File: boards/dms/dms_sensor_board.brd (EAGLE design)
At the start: 49.5 x 44.5 mm, 33 parts, among them Q1 IRLML5203, Q2 IRLML5203, Q3 IRLML5203, Q4 IRLML5203

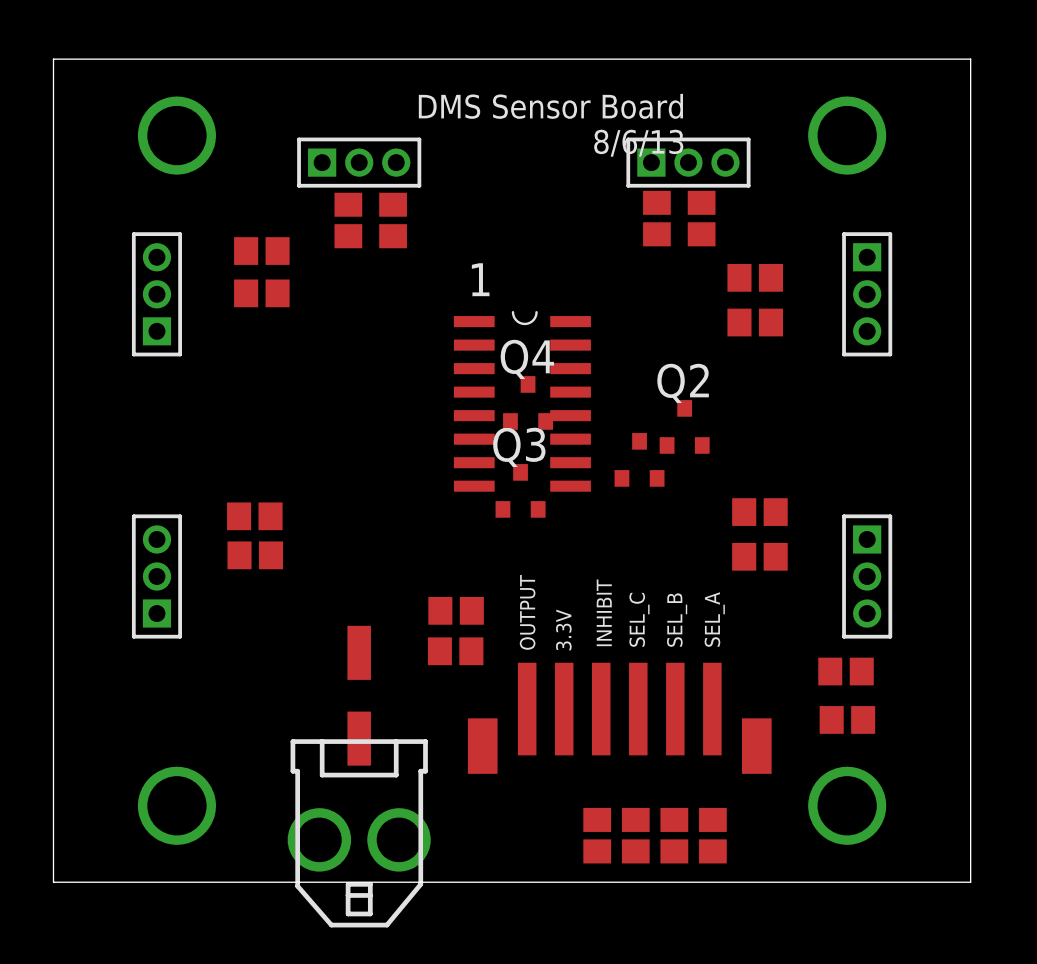
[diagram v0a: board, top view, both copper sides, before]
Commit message: changes for new boards, cleared DRC
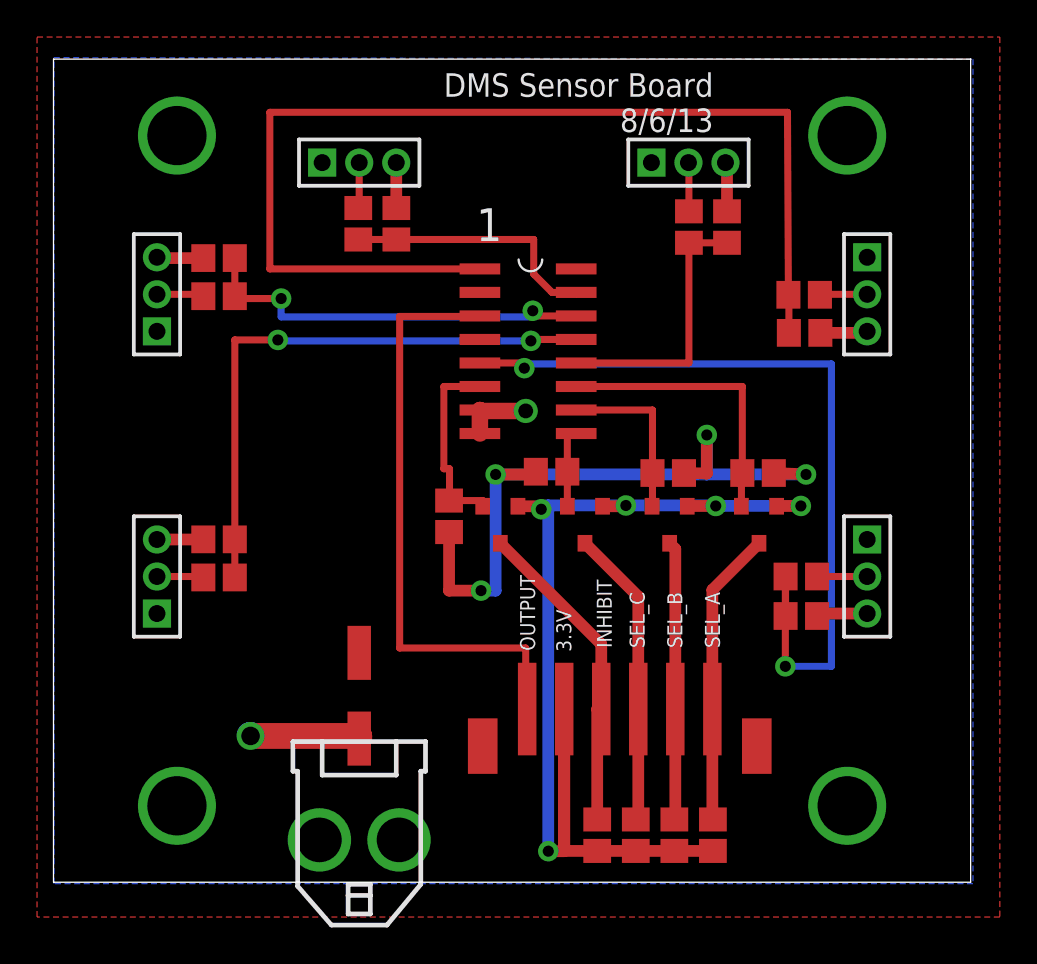
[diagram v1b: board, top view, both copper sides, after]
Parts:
- moved R19 24.2 mm to (18.8, 19.8), turned to 90 degrees
- moved R17 19.2 mm to (24.4, 22.2)
- moved R13 17.9 mm to (35.5, 22.1), turned to 180 degrees
- moved R15 15.0 mm to (30.7, 22.1), turned to 180 degrees
- moved Q1 7.34 mm to (35.6, 19.3), turned to 180 degrees
- moved Q4 6.75 mm to (21.6, 19.3), turned to 180 degrees
- moved Q2 5.35 mm to (30.7, 19.3), turned to 180 degrees
- moved R11 4.14 mm to (37.8, 16.5)
- moved Q3 3.93 mm to (26.2, 19.3), turned to 180 degrees
- moved R12 3.90 mm to (37.8, 14.4)
- moved MUX1 2.86 mm to (23.1, 28.7)
- moved R9 2.80 mm to (38.0, 31.7)
- moved R10 2.72 mm to (38.0, 29.7)
- moved R4 2.34 mm to (6.40, 33.7)
- moved R3 2.32 mm to (6.40, 31.6)
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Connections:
- removed net N$1: MUX1.2
- removed net N_GND: MUX1.16, MUX1.4
- net 5V: now also MUX1.16
- net A_H: now also MUX1.11
- net B_H: now also MUX1.10
- net C_H: now also MUX1.9
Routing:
- net 3VCC: track 0.00 -> 63.2 mm, vias 0 -> 5
- net DATA5-L: track 0.00 -> 59.7 mm
- net DATA6-L: track 0.00 -> 45.3 mm, vias 0 -> 2
- net 5V: track 0.00 -> 38.5 mm, vias 0 -> 4
- net N$5: track 0.00 -> 32.5 mm
- net DATA1-L: track 0.00 -> 31.4 mm, vias 0 -> 2
- net GND: track 0.00 -> 25.7 mm, vias 0 -> 2
- net DATA2-L: track 0.00 -> 22.2 mm, vias 0 -> 2
- net INHIBIT: track 0.00 -> 17.4 mm
- net SEL_C: track 0.00 -> 16.2 mm
- net SEL_A: track 0.00 -> 16.0 mm
- net A_H: track 0.00 -> 15.4 mm
- net SEL_B: track 0.00 -> 15.1 mm
- net DATA4-L: track 0.00 -> 14.6 mm
- net DATA3-L: track 0.00 -> 14.1 mm
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- added copper zone on layer 1, net 5V
- added copper zone on layer 16, net GND
